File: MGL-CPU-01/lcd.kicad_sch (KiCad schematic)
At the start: 34 parts, among them P2 LCD FPC, Q1 2SA1576A, U4 IR3E02

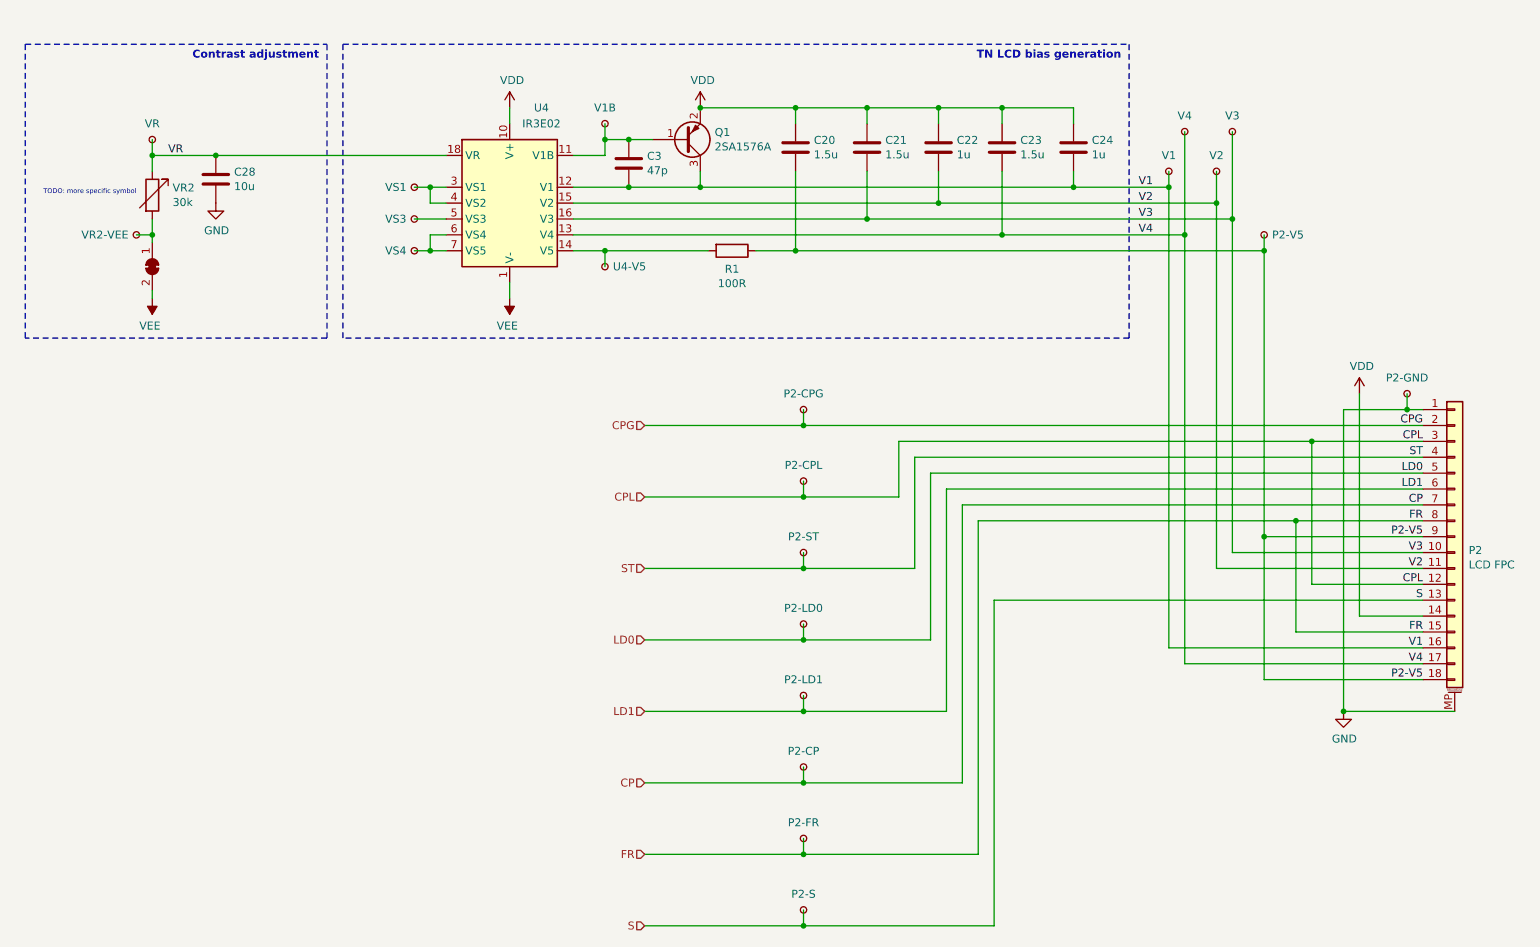
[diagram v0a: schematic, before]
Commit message: Tidy up potentiometer symbols, add contrast pot symbols
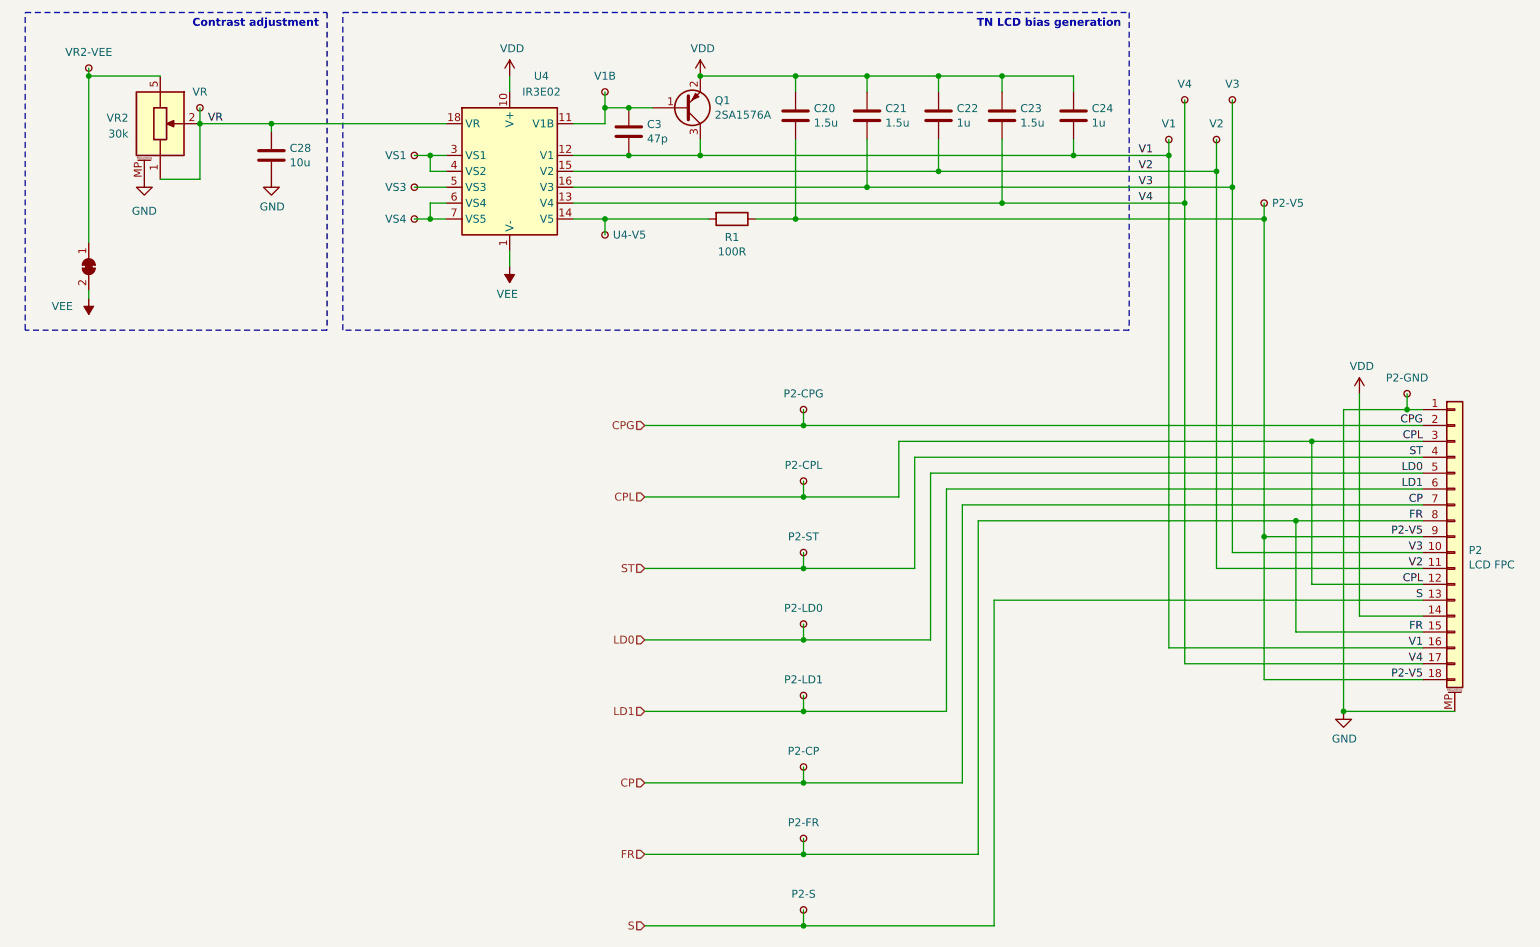
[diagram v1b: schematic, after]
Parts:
- removed VR2: 30k, symbol Device:R_Variable
- added VR2: 30k, symbol Gekkio_Device_Specialized:R_Potentiometer_GameBoy_Contrast_MGB
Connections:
- net GND: now also VR2.MP (MountPin)
- net VR: now also VR2.1 (4), VR2.2
- net at JP1.1 (A), TP64.1: now also VR2.5
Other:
- note removed: "TODO: more specific symbol"
- moved on the sheet: C20, C21, C22, C23, C24, C3, Q1, R1, U4
